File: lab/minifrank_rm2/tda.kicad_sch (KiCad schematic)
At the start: 6 parts, among them U3 TDA1387T

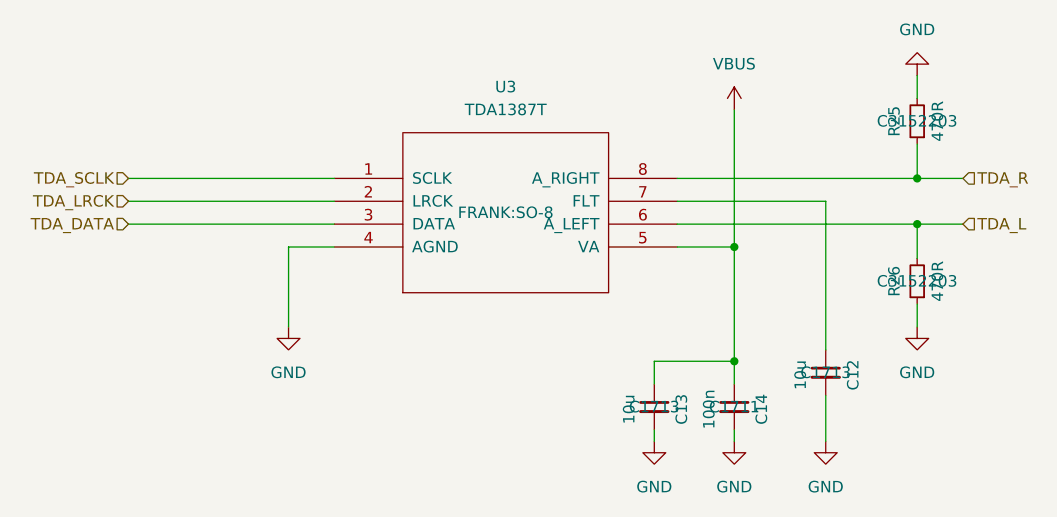
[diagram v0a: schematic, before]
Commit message: MiniFRANK RM2 1.02
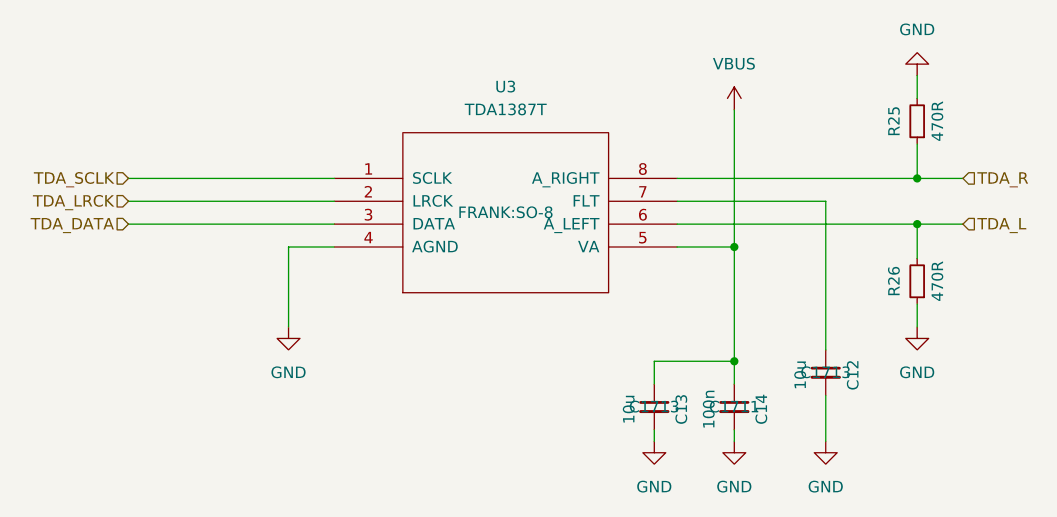
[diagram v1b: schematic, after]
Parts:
- R25, R26: LCSC C3152203 -> (none)
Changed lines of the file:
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@@
 			)
 		)
-		(property "LCSC" "C3152203"
+		(property "LCSC" ""
 			(at 186.69 101.6 0)
 			(effects
@@
 			)
 		)
-		(property "LCSC" "C3152203"
-			(at 186.69 83.82 0)
-			(effects
+		(property "LCSC" ""
+			(at 186.69 83.82 0)
+			(effects
